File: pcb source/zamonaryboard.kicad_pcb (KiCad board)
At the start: 2 copper layers, 52.3 x 40.6 mm, 11 parts, among them J1 USB_C_Receptacle_USB2.0_14P, U1 CH32V003JxMx, U2 ME6211C33M5

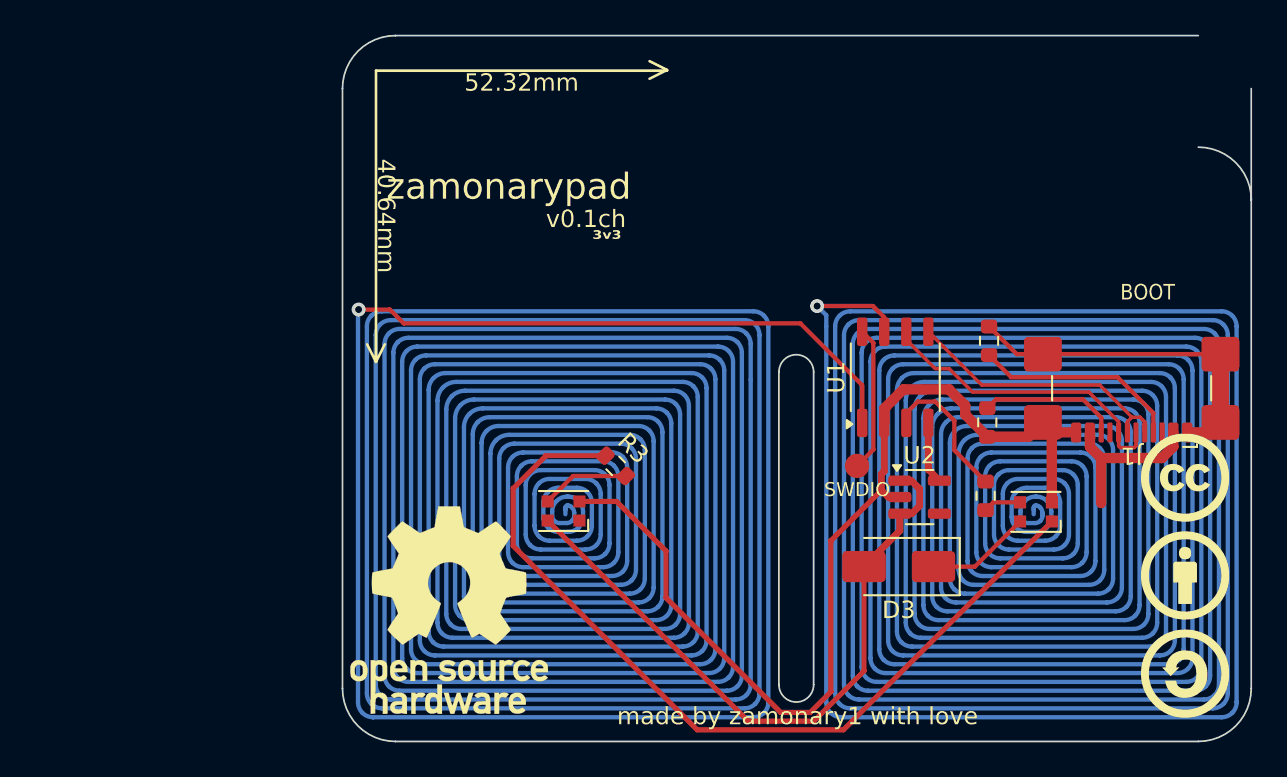
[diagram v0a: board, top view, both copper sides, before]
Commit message: Working pcb
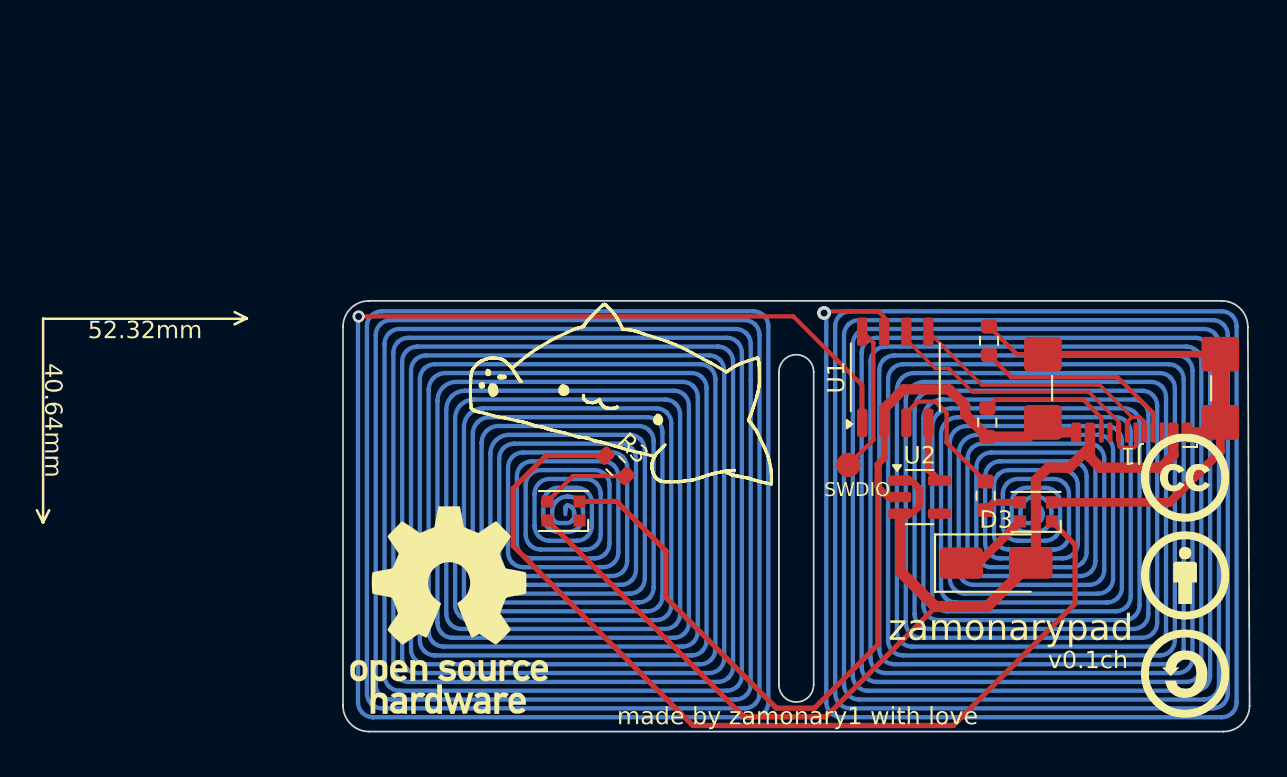
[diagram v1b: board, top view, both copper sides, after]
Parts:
- moved D3 5.60 mm to (156.5, 102.0), turned to 0 degrees
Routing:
- net VBUS: track 47.3 -> 62.8 mm
- net GND: track 77.8 -> 86.4 mm
- net Net-(D1-DOUT): track 49.8 -> 54.2 mm
- net Net-(D1-VDD): track 6.06 -> 4.38 mm
- net BTN2: track 1103.8 -> 1102.8 mm
- net BTN1: track 1131.4 -> 1130.9 mm
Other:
- board size 52.3 x 40.6 mm -> 52.2 x 24.8 mm
- board text removed: "3v3"
- board text removed: "BOOT"
